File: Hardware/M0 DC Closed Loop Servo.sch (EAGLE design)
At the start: 56 parts, among them Q1 2N7002PW, Q2 2.5A/30V, U1 DRV8871, U2 DRV8871, U3 ATSAMD21G-A, U4 3.3V, U5 74AHC1G125, U6 EEPROM-I2CSMD, Y1 32.768kHz

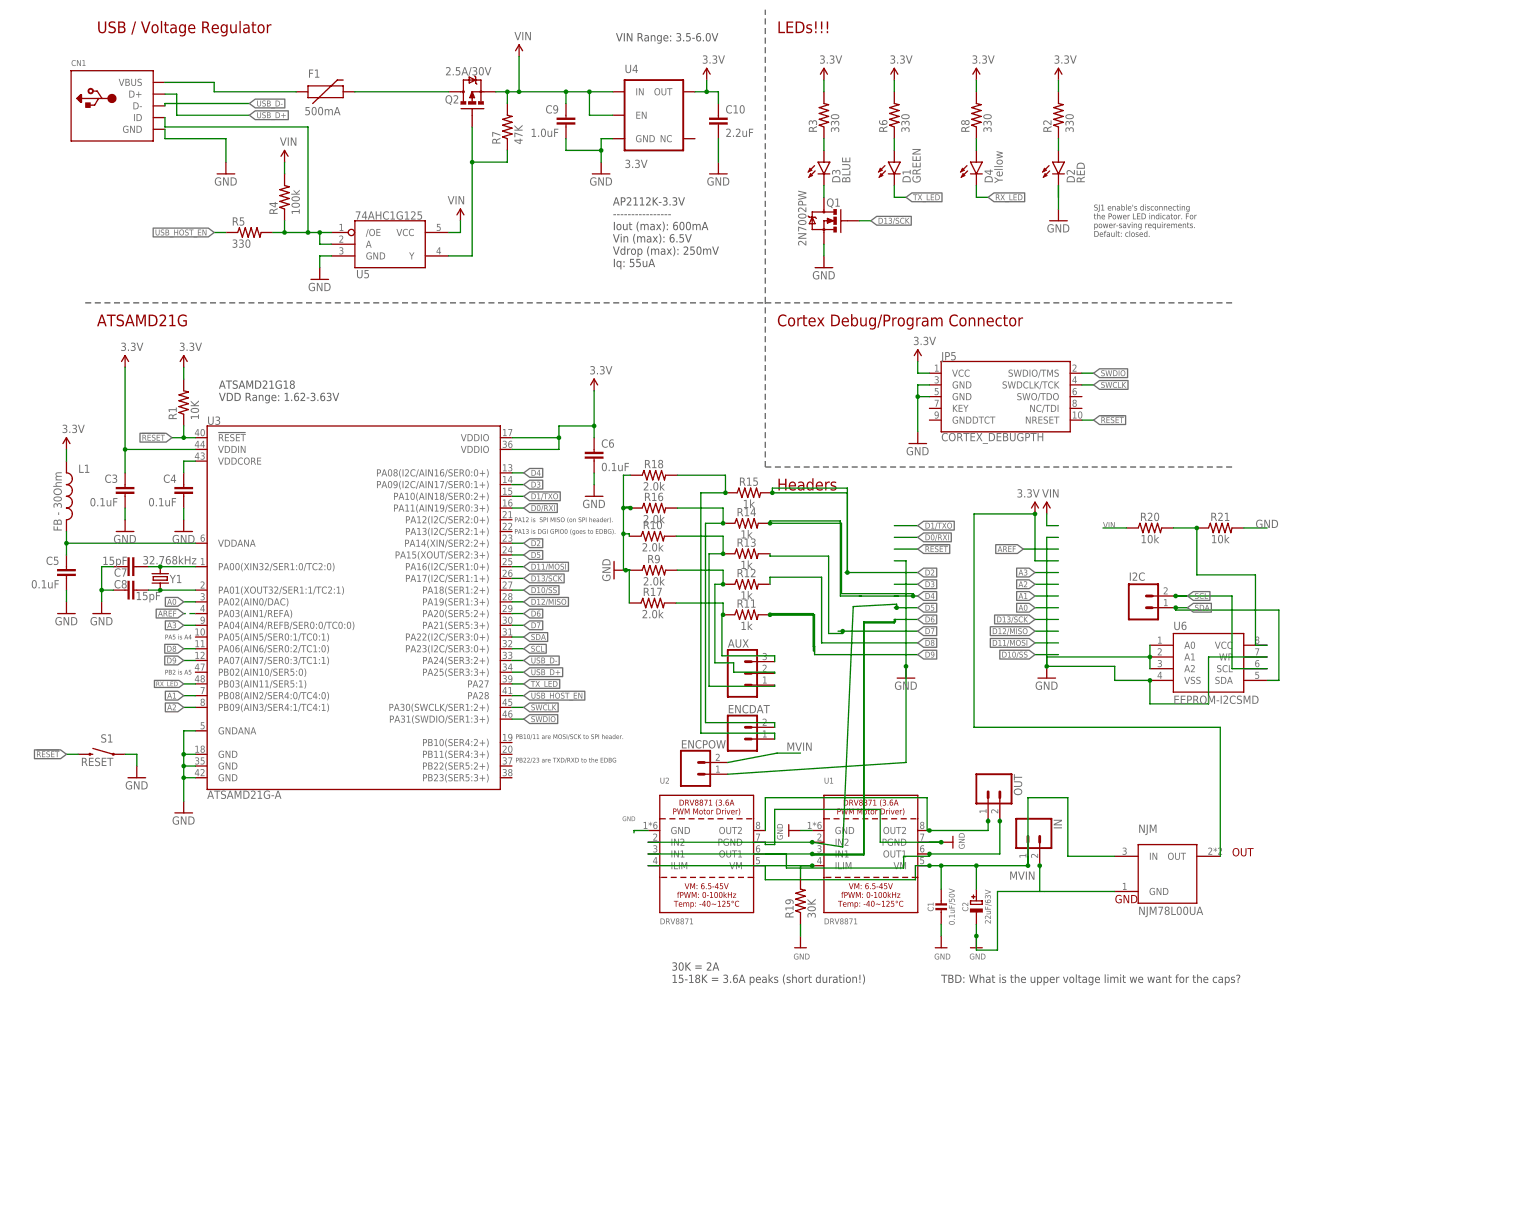
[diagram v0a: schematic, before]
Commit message: COMPLETE OVER HULL
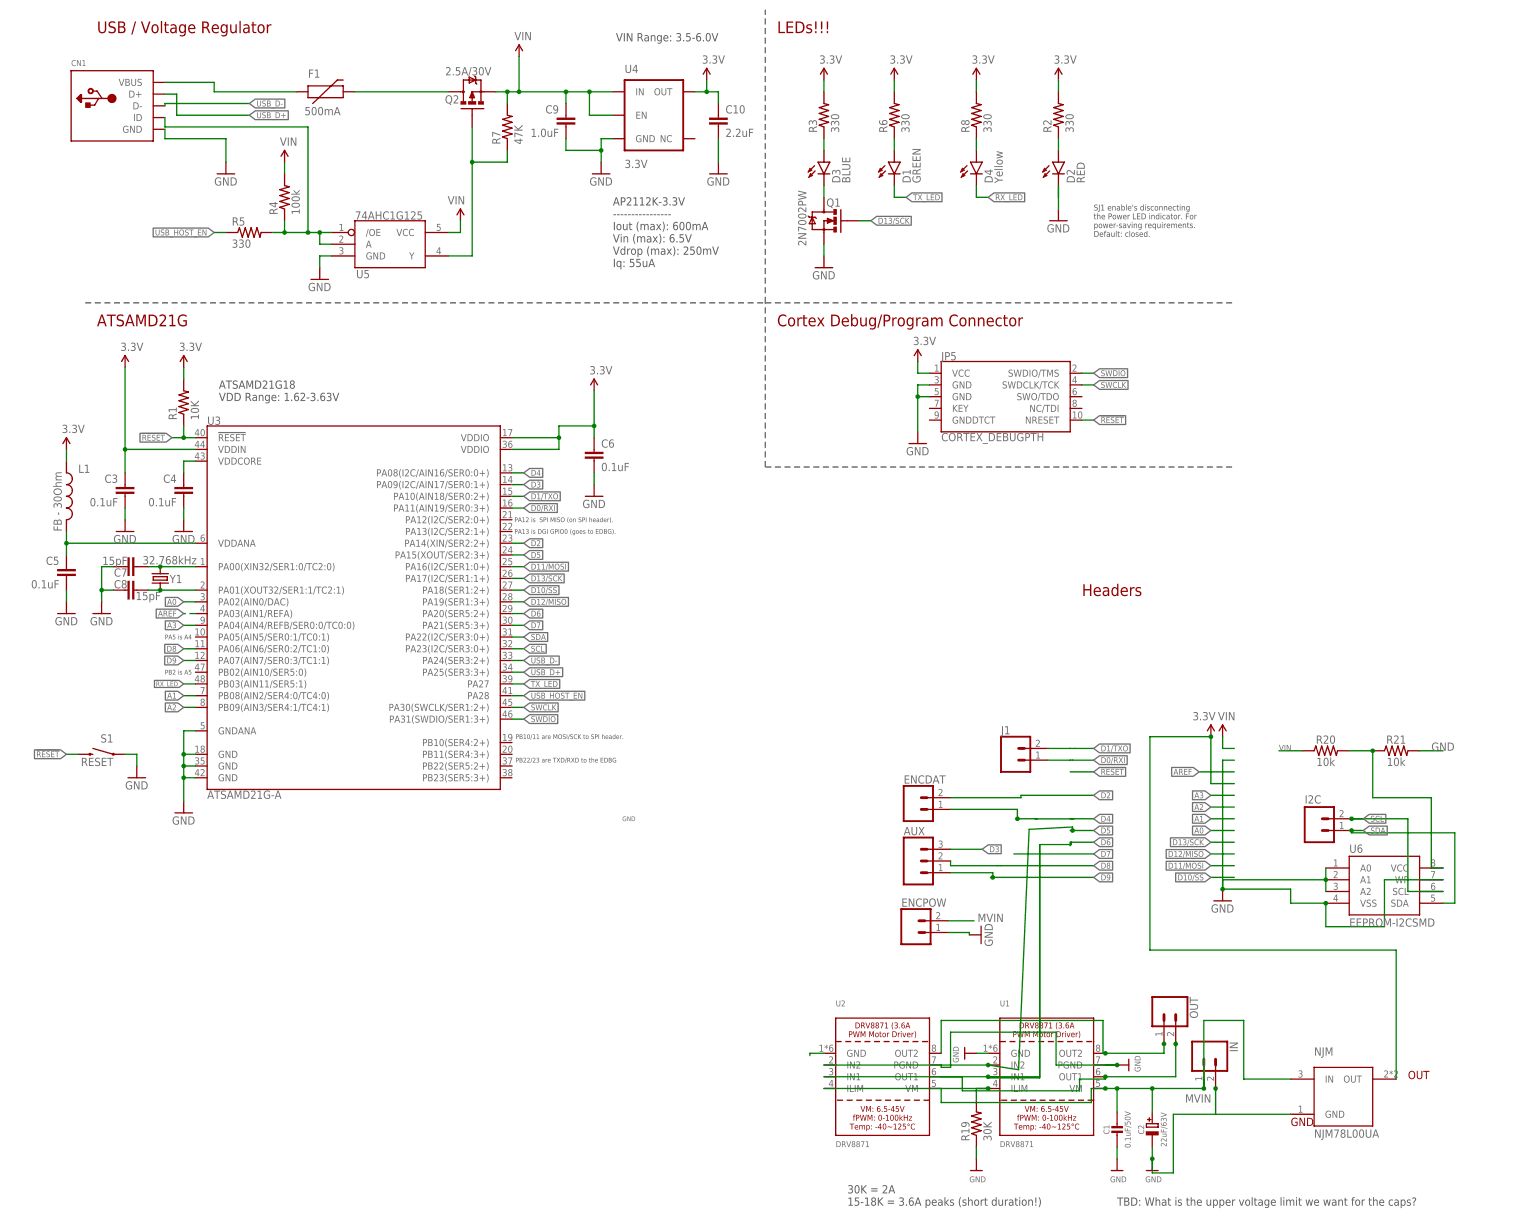
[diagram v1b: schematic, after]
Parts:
- removed R10, R16, R17, R18, R9: 2.0k, SparkFun-Resistors:2.0KOHM-0603-1/10W-5%
- removed R11, R12, R13, R14, R15: 1k, SparkFun-Resistors:1KOHM-0603-1/10W-1%
- added J1: (no value), SparkFun-Connectors:CONN_02
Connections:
- removed net ENCODER: ENCDAT.1, R15.1, R18.2
- removed net N$14: AUX.3, R11.1, R17.2
- removed net N$16: AUX.2, R12.1, R9.2
- removed net N$17: AUX.1, R10.2, R13.1
- removed net N$18: ENCDAT.2, R14.1, R16.2
- net D0/RXI: now also J1.1
- net D1/TXO: now also J1.2
- net D2: now also ENCDAT.2; no longer R15.2
- net D3: now also AUX.3
- net D4: now also ENCDAT.1; no longer R14.2
- net D7: no longer R13.2
- net D8: now also AUX.2; no longer R12.2
- net D9: now also AUX.1; no longer R11.2
- net GND: no longer R10.1, R16.1, R17.1, R18.1, R9.1
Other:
- moved on the sheet: AUX, C1, C2, ENCDAT, ENCPOW, I2C, IN, NJM, OUT, R19, R20, R21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
